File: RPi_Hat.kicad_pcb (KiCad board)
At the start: 2 copper layers, 120 x 75 mm, 112 parts, among them J1 Barrel_Jack, J10 Audio-Jack-3, J11 Screw_Terminal_1x03, J12 Screw_Terminal_1x03, J13 Screw_Terminal_1x03, J14 Screw_Terminal_1x03, J15 Screw_Terminal_1x03, J16 Screw_Terminal_1x03, J17 Screw_Terminal_1x03, J18 Screw_Terminal_1x03, J2 Audio-Jack-3, J3 Audio-Jack-3, J300 RPi_GPIO, J4 Audio-Jack-3, J5 Audio-Jack-3, J6 Audio-Jack-3, J7 Audio-Jack-3, J8 Audio-Jack-3, J9 Audio-Jack-3, Q1 TSM3404, Q2 TSM3404, Q3 TSM3404, Q4 TSM3404, Q5 TSM3404, Q6 TSM3404, Q7 TSM3404, Q8 TSM3404, U1 EL817S1(B)(TU)-F, U2 EL817S1(B)(TU)-F, U3 EL817S1(B)(TU)-F, U4 EL817S1(B)(TU)-F, U5 EL817S1(B)(TU)-F, U6 EL817S1(B)(TU)-F, U7 EL817S1(B)(TU)-F, U8 EL817S1(B)(TU)-F

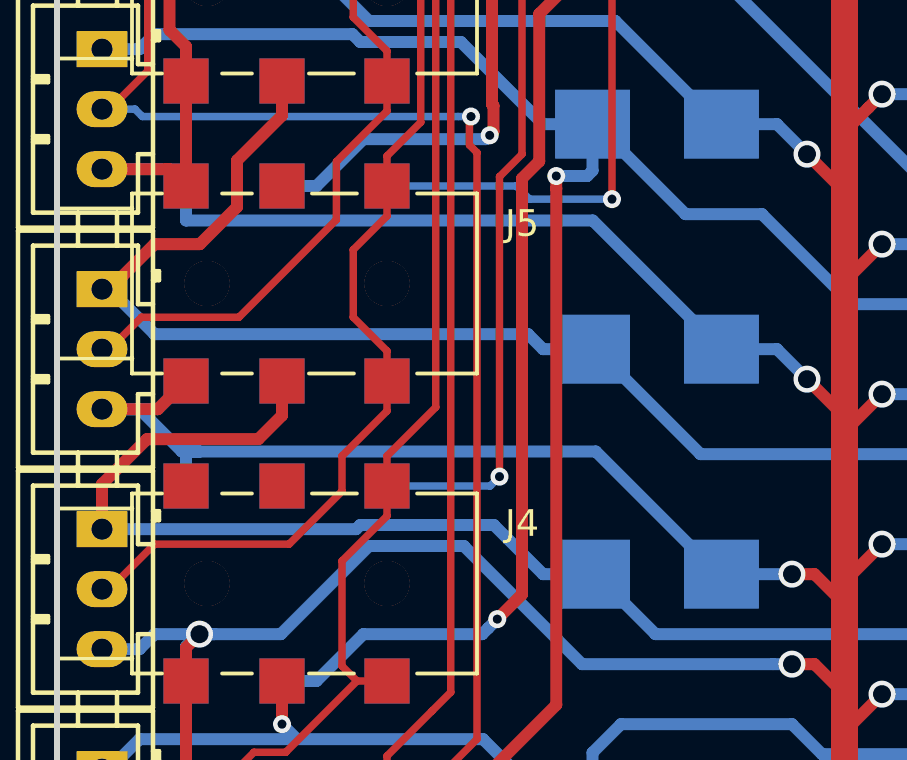
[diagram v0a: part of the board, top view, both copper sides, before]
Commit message: final PCB as ordered
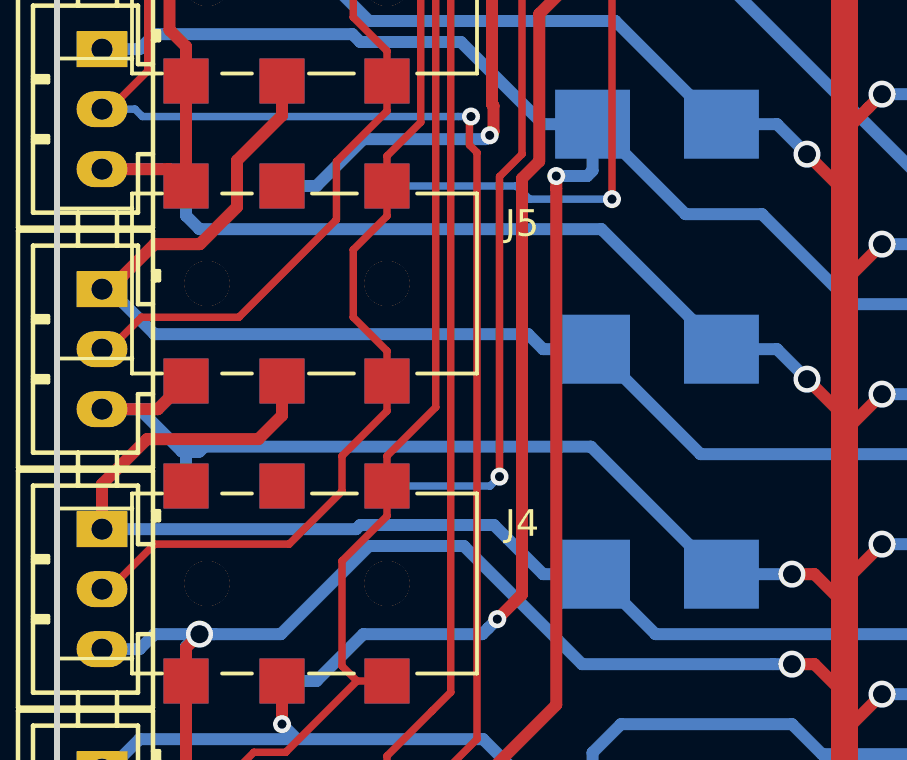
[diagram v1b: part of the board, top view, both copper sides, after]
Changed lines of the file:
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@@
 (kicad_pcb (version 20170123) (host pcbnew "(2017-06-12 revision 19d5cc754)-master")
   (general
-    (links 0)
-    (no_connects 19)
+    (links 239)
+    (no_connects 18)
     (area -37.550001 -15.7 134.078571 69.4825)
     (thickness 1.6)
     (drawings 69)
-    (tracks 962)
+    (tracks 964)
     (zones 0)
     (modules 112)
@@
     (trace_clearance 0.25)
     (zone_clearance 0.508)
-    (zone_45_only no)
+    (zone_45_only yes)
     (trace_min 0.15)
     (segment_width 0.1)
@@
     (pad_to_mask_clearance 0)
     (aux_axis_origin 0 0)
-    (grid_origin 74 -5)
+    (grid_origin 89 32.25)
     (visible_elements 7FFFFFFF)
     (pcbplotparams
-      (layerselection 0x00030_80000001)
-      (usegerberextensions false)
+      (layerselection 0x010f0_ffffffff)
+      (usegerberextensions true)
       (excludeedgelayer true)
       (linewidth 0.100000)
@@
   (segment (start 13.5 -0.5) (end 13.5 2.68) (width 0.9) (layer B.Cu) (net 2))
   (segment (start 13.5 2.68) (end 13.45 2.73) (width 0.9) (layer B.Cu) (net 2))
+  (segment (start -23.2 22.06151) (end -23.2 23.05) (width 0.4) (layer B.Cu) (net 3))
+  (segment (start -23.2 23.05) (end -22.75 23.5) (width 0.4) (layer B.Cu) (net 3))
+  (segment (start -22.75 23.5) (end -9.35116 23.5) (width 0.4) (layer B.Cu) (net 3))
+  (segment (start -9.35116 23.5) (end -5.35116 27.5) (width 0.4) (layer B.Cu) (net 3))
+  (segment (start -22.75 30.911509) (end -22.588491 30.75) (width 0.4) (layer B.Cu) (net 3))
+  (segment (start -22.588491 30.75) (end -9.70022 30.75) (width 0.4) (layer B.Cu) (net 3))
+  (segment (start -9.70022 30.75) (end -5.45022 35) (width 0.4) (layer B.Cu) (net 3))
+  (segment (start -5.45022 35) (end -5.35116 35) (width 0.4) (layer B.Cu) (net 3))
   (segment (start -23.2 38.56151) (end -23.2 37.45) (width 0.4) (layer F.Cu) (net 3))
   (segment (start -23.2 37.45) (end -22.75 37) (width 0.4) (layer F.Cu) (net 3))
@@
   (segment (start -22.78849 37) (end -22.25 37) (width 0.4) (layer B.Cu) (net 3))
   (segment (start -23.338491 30.911509) (end -22.75 30.911509) (width 0.4) (layer B.Cu) (net 3))
-  (segment (start -22.75 30.911509) (end -9.538711 30.911509) (width 0.4) (layer B.Cu) (net 3))
   (segment (start -23.2 32.06151) (end -23.199999 30.911509) (width 0.4) (layer B.Cu) (net 3))
   (segment (start -23.199999 30.911509) (end -22.75 30.911509) (width 0.4) (layer B.Cu) (net 3))
@@
   (segment (start -15.35116 5) (end -13.70148 5) (width 0.4) (layer B.Cu) (net 3))
   (segment (start -13.70148 5) (end -11.70148 7) (width 0.4) (layer B.Cu) (net 3))
-  (segment (start -23.2 22.06151) (end -23.199999 23.211511) (width 0.4) (layer B.Cu) (net 3))
-  (segment (start -23.199999 23.211511) (end -9.639649 23.211511) (width 0.4) (layer B.Cu) (net 3))
-  (segment (start -9.639649 23.211511) (end -5.35116 27.5) (width 0.4) (layer B.Cu) (net 3))
   (segment (start -26 21.5) (end -23.76151 21.5) (width 0.4) (layer B.Cu) (net 3))
   (segment (start -23.76151 21.5) (end -23.2 22.06151) (width 0.4) (layer B.Cu) (net 3))
   (segment (start -26 29.5) (end -24.75 29.5) (width 0.4) (layer B.Cu) (net 3))
   (segment (start -24.75 29.5) (end -23.338491 30.911509) (width 0.4) (layer B.Cu) (net 3))
-  (segment (start -9.538711 30.911509) (end -5.45022 35) (width 0.4) (layer B.Cu) (net 3))
-  (segment (start -5.45022 35) (end -5.35116 35) (width 0.4) (layer B.Cu) (net 3))
   (segment (start -9.95022 47) (end -5.45022 42.5) (width 0.4) (layer B.Cu) (net 3))
   (segment (start -5.45022 42.5) (end -5.35116 42.5) (width 0.4) (layer B.Cu) (net 3))
@@
     (connect_pads (clearance 0.508))
     (min_thickness 0.254)
-    (keepout (tracks not_allowed) (vias not_allowed) (copperpour allowed))
+    (keepout (tracks not_allowed) (vias not_allowed) (copperpour not_allowed))
     (fill (arc_segments 16) (thermal_gap 0.508) (thermal_bridge_width 0.508))
     (polygon
       (pts
-        (xy 31 -10.5) (xy 31 -6.5) (xy 32.5 -6.5) (xy 32.5 -11) (xy 31 -11)
+        (xy 40.75 -7.75) (xy 40.75 -3.75) (xy 42.25 -3.75) (xy 42.25 -8.25) (xy 40.75 -8.25)
       )
     )
